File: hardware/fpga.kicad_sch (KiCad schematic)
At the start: 1 part, among them U1 XC7A75T-FGG676

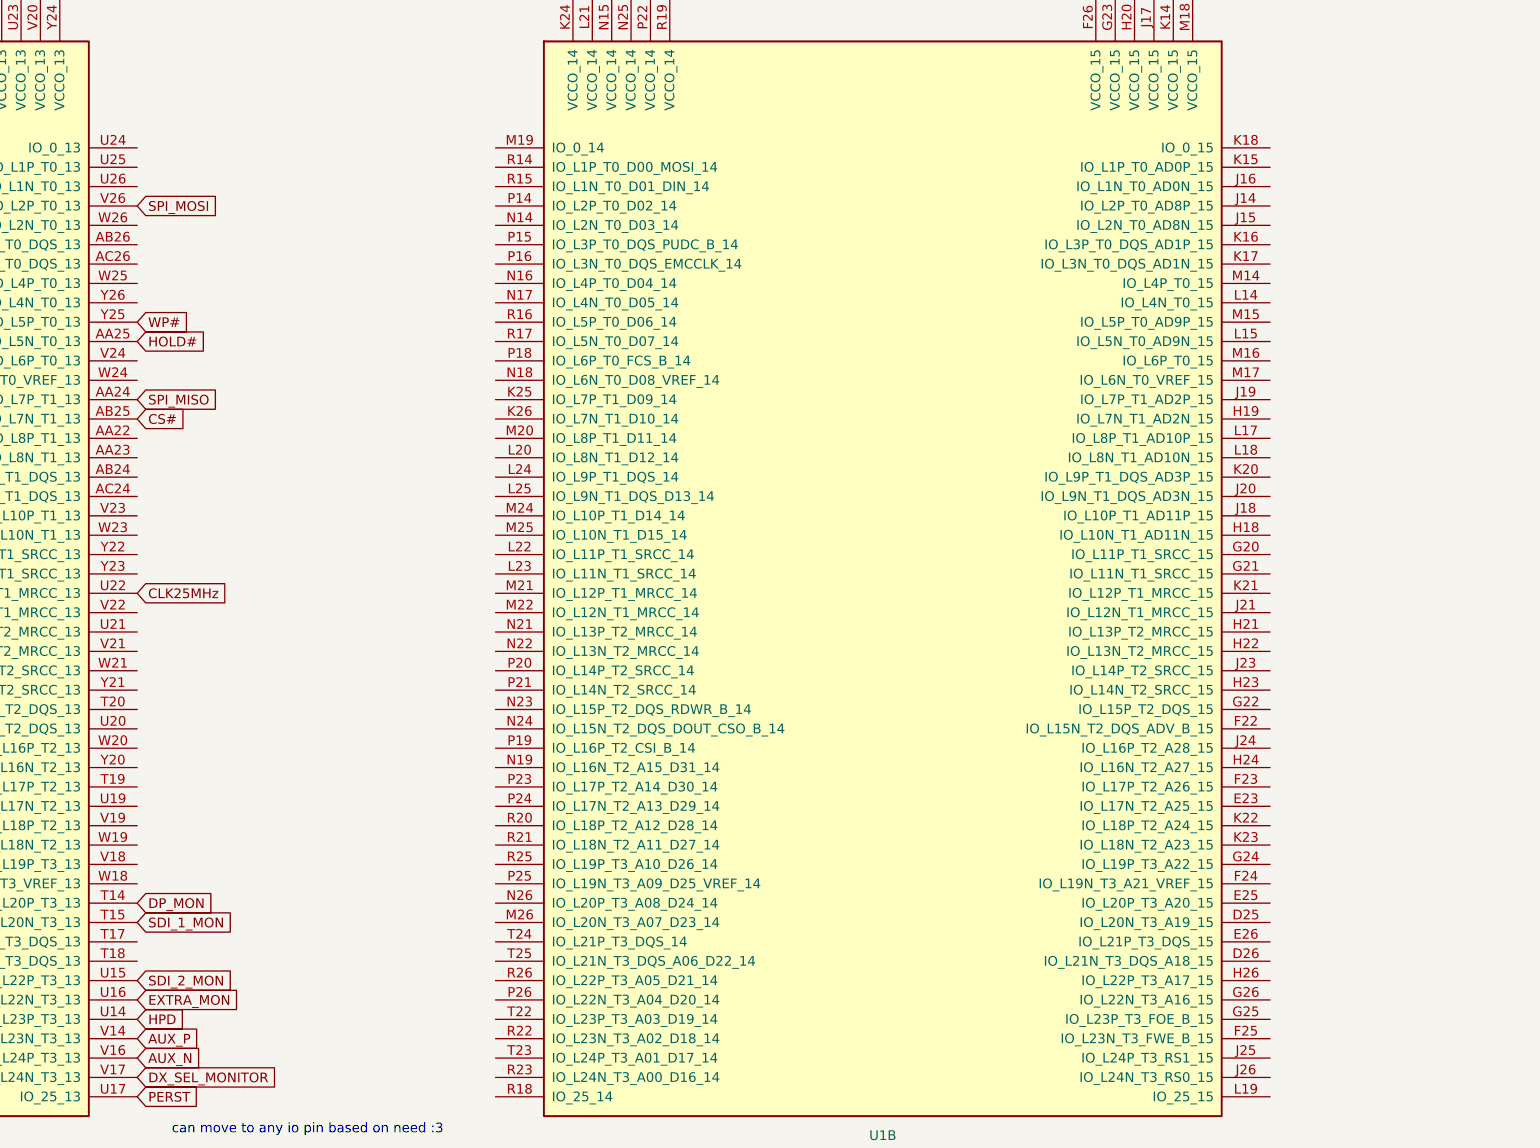
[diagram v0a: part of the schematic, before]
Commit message: finished pcb
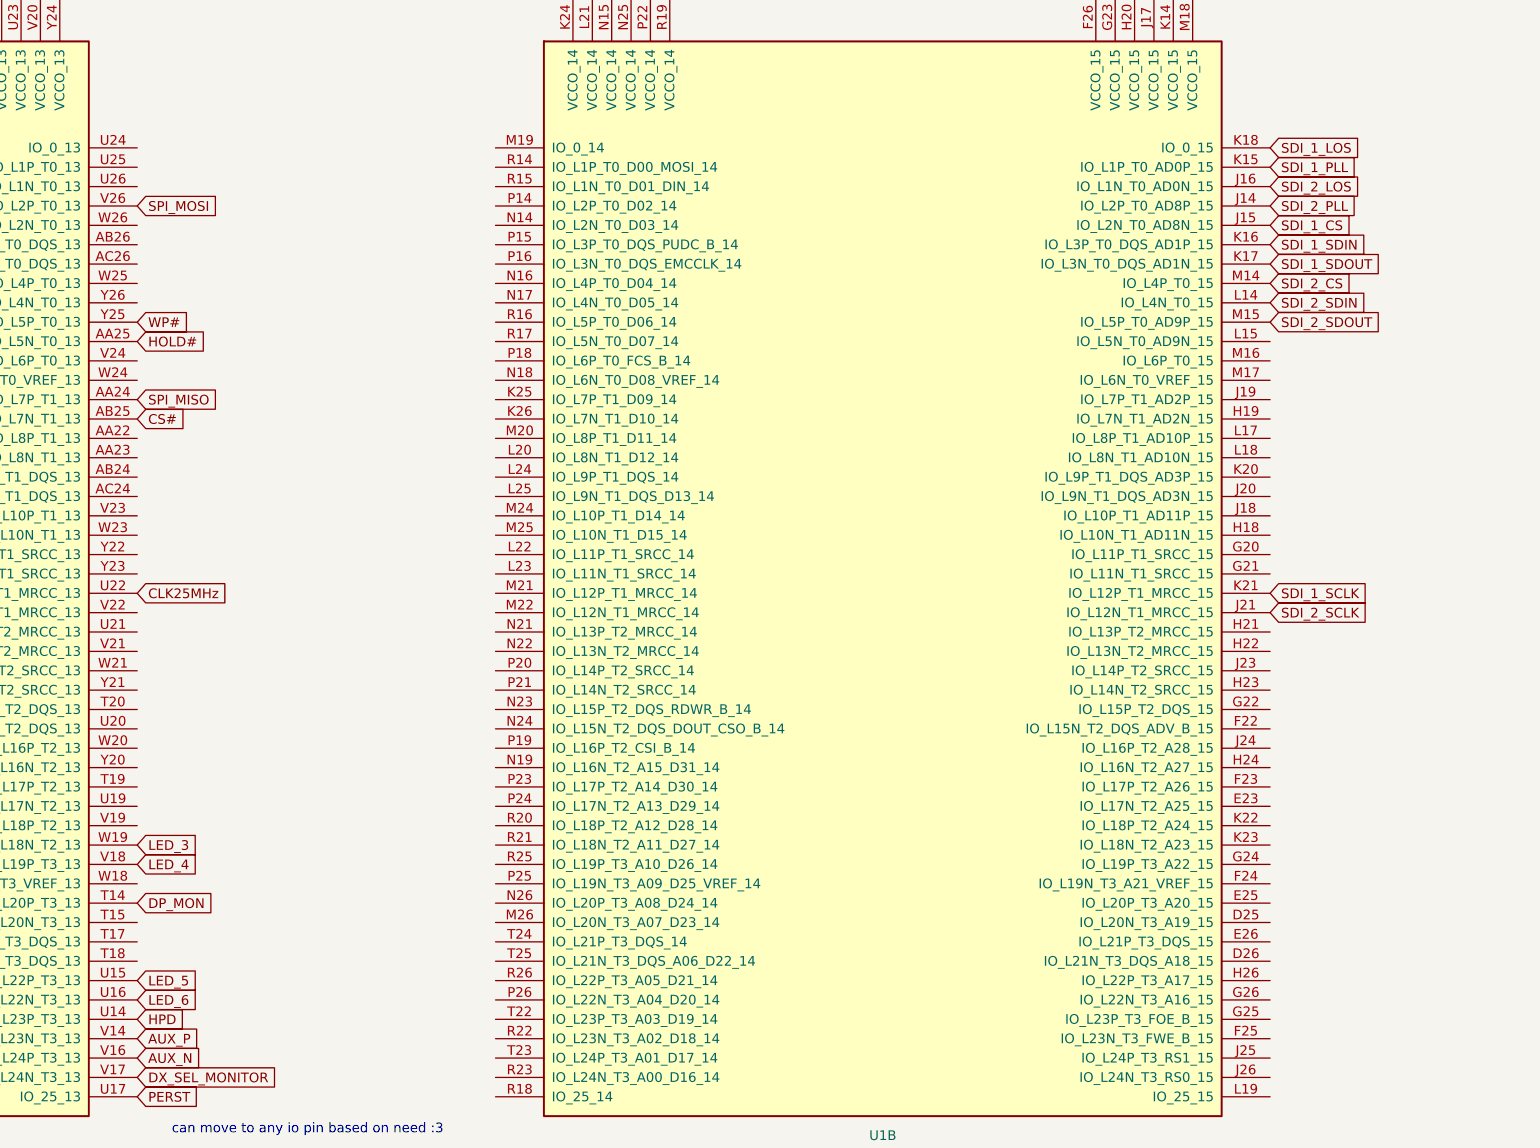
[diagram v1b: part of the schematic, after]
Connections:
- net LED_4: now reaches U1.V18 (IO_L19P_T3_13)
- net LED_3: now reaches U1.W19 (IO_L18N_T2_13)
- net SDI_2_PLL: now reaches U1.J14 (IO_L2P_T0_AD8P_15)
- net SDI_1_CS: now reaches U1.J15 (IO_L2N_T0_AD8N_15)
- net SDI_2_LOS: now reaches U1.J16 (IO_L1N_T0_AD0N_15)
- net SDI_2_SCLK: now reaches U1.J21 (IO_L12N_T1_MRCC_15)
- net SDI_1_PLL: now reaches U1.K15 (IO_L1P_T0_AD0P_15)
- net SDI_1_SDIN: now reaches U1.K16 (IO_L3P_T0_DQS_AD1P_15)
- net SDI_1_SDOUT: now reaches U1.K17 (IO_L3N_T0_DQS_AD1N_15)
- net SDI_1_LOS: now reaches U1.K18 (IO_0_15)
- net SDI_1_SCLK: now reaches U1.K21 (IO_L12P_T1_MRCC_15)
- net SDI_2_SDIN: now reaches U1.L14 (IO_L4N_T0_15)
- net SDI_2_CS: now reaches U1.M14 (IO_L4P_T0_15)
- net SDI_2_SDOUT: now reaches U1.M15 (IO_L5P_T0_AD9P_15)
- net EXTRA_MON renamed LED_6
- net SDI_1_MON: no longer names the net of U1.T15 (IO_L20N_T3_13)
- net SDI_2_MON renamed LED_5

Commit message: added changed
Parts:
- U1: Arrow Price/Stock (none) -> $77.7344
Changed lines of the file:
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@@
+			)
+		)
+		(property "Arrow Price/Stock" "$77.7344"
+			(at 67.31 120.65 0)
+			(hide yes)
+			(show_name no)
+			(do_not_autoplace no)
+			(effects
+				(font
+					(size 1.27 1.27)
+				)
 			)
 		)
@@
 			)
 		)
+		(property "Arrow Price/Stock" "$77.7344"
+			(at 215.9 120.65 0)
+			(hide yes)
+			(show_name no)
+			(do_not_autoplace no)
+			(effects
+				(font
+					(size 1.27 1.27)
+				)
+			)
+		)
 		(pin "B18"
 		)
@@
 			(at 365.76 120.65 0)
 			(hide yes)
+			(show_name no)
+			(do_not_autoplace no)
+			(effects
+				(font
+					(size 1.27 1.27)
+				)
+			)
+		)
+		(property "Arrow Price/Stock" "$77.7344"
+			(at 365.76 120.65 0)
+			(hide yes)
